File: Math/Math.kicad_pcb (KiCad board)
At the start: 2 copper layers, 100 x 100 mm, 6 parts, among them J1 Buss, U1 AM9511A, U2 74LS85, U3 74LS04, U4 74LS30

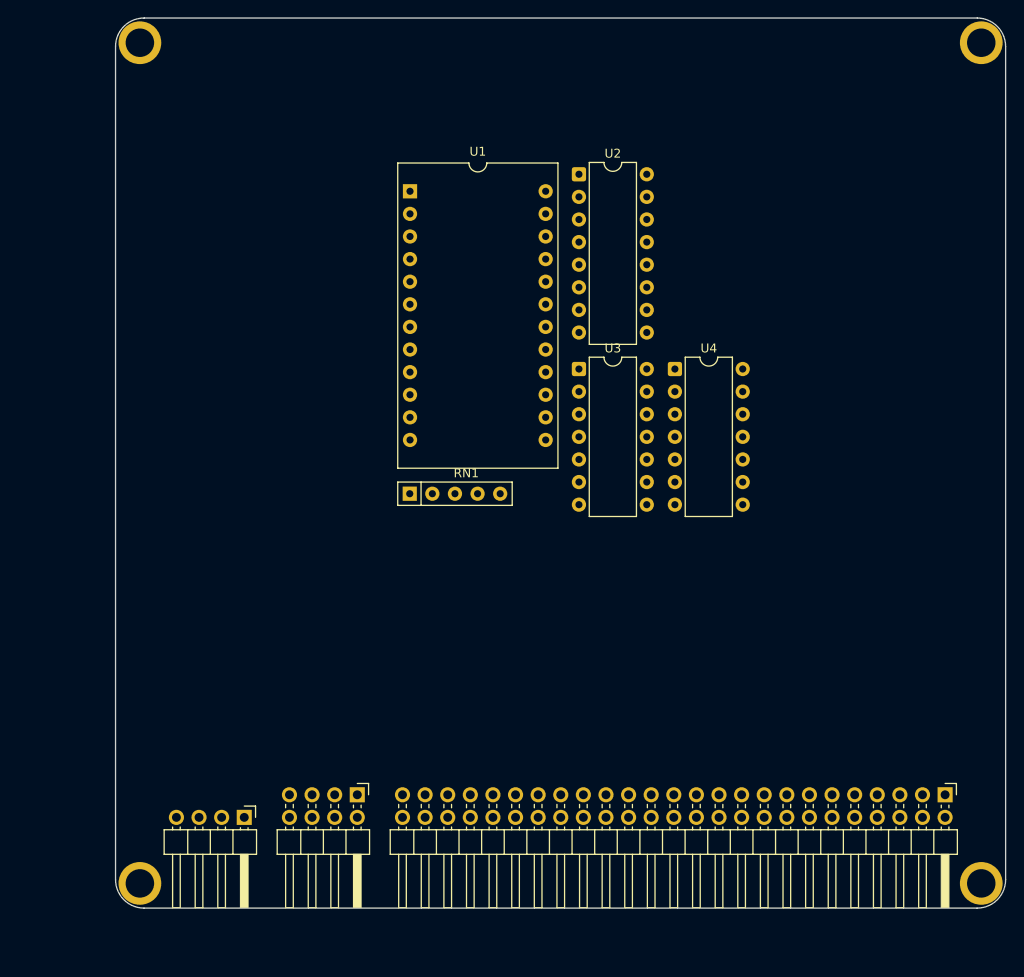
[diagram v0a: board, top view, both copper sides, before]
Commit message: mainly actually saving out vs.code along with sorting out the math card
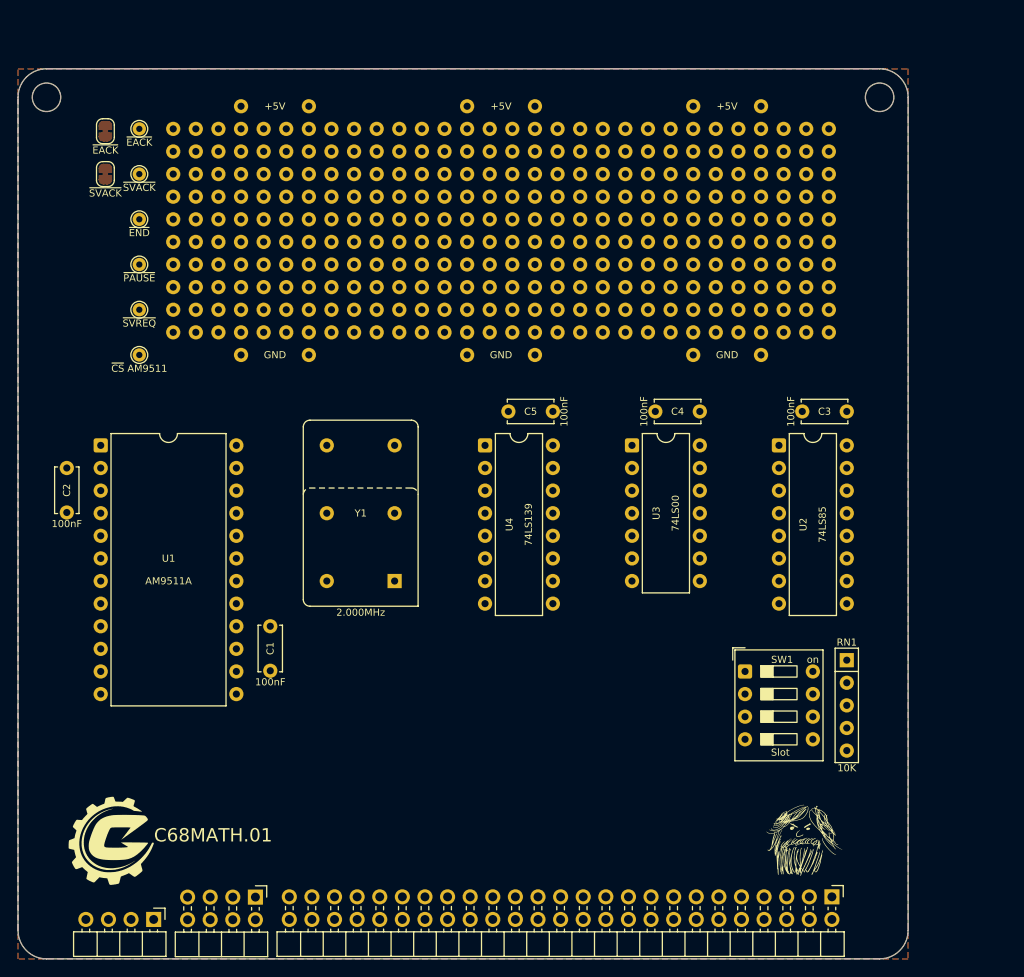
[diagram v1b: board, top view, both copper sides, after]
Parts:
- added C1: 100nF, 0-Footprints:C_Disc_D5.0mm_W2.5mm_P5.00mm, F.Cu at (53.3, 87.6)
- added C2: 100nF, 0-Footprints:C_Disc_D5.0mm_W2.5mm_P5.00mm, F.Cu at (30.5, 69.8)
- added C3: 100nF, 0-Footprints:C_Disc_D5.0mm_W2.5mm_P5.00mm, F.Cu at (118.1, 63.5)
- added C4: 100nF, 0-Footprints:C_Disc_D5.0mm_W2.5mm_P5.00mm, F.Cu at (101.6, 63.5)
- added C5: 100nF, 0-Footprints:C_Disc_D5.0mm_W2.5mm_P5.00mm, F.Cu at (80.1, 63.5)
- added G1: Logo, 0-Footprints:Crank, F.Cu at (35.6, 111.8)
- added G2: Logo, 0-Footprints:crankery_small, F.Cu at (113.0, 111.8)
- added JP1: ~{EACK}, 0-Footprints:SolderJumper-2_P1.3mm_Bridged_RoundedPad1.0x1.5mm, F.Cu at (34.8, 32.0)
- added JP2: ~{SVACK}, 0-Footprints:SolderJumper-2_P1.3mm_Bridged_RoundedPad1.0x1.5mm, F.Cu at (34.8, 36.8)
- added QC1: Grid, 0-Footprints:Grid, F.Cu at (42.4, 29.2)
- added QC2: Grid, 0-Footprints:Grid, F.Cu at (67.8, 29.2)
- added QC3: Grid, 0-Footprints:Grid, F.Cu at (93.2, 29.2)
- added SW1: Slot, 0-Footprints:SW_DIP_SPSTx04_Slide_9.78x12.34mm_W7.62mm_P2.54mm, F.Cu at (106.7, 92.7)
- added TP1: ~{EACK}, 0-Footprints:TestPoint_THTPad_D1.5mm_Drill0.7mm, F.Cu at (38.6, 31.8)
- added TP2: ~{SVACK}, 0-Footprints:TestPoint_THTPad_D1.5mm_Drill0.7mm, F.Cu at (38.6, 36.8)
- added TP3: ~{END}, 0-Footprints:TestPoint_THTPad_D1.5mm_Drill0.7mm, F.Cu at (38.6, 41.9)
- added TP4: ~{PAUSE}, 0-Footprints:TestPoint_THTPad_D1.5mm_Drill0.7mm, F.Cu at (38.6, 47.0)
- added TP5: ~{SVREQ}, 0-Footprints:TestPoint_THTPad_D1.5mm_Drill0.7mm, F.Cu at (38.6, 52.1)
- added TP6: ~{CS} AM9511, 0-Footprints:TestPoint_THTPad_D1.5mm_Drill0.7mm, F.Cu at (38.6, 57.1)
- added Y1: 2.000MHz, 0-Footprints:Oscillator_DIP-14, F.Cu at (67.3, 82.5)
- RN1: footprint Resistor_THT:R_Array_SIP5 -> 0-Footprints:R_Array_SIP5
- U1: footprint Package_DIP:DIP-24_18.0mmx34.29mm_W15.24mm -> 0-Footprints:DIP-24_W15.24mm
- U2: footprint Package_DIP:DIP-16_W7.62mm -> 0-Footprints:DIP-16_W7.62mm
- U3: value 74LS04 -> 74LS00; footprint Package_DIP:DIP-14_W7.62mm -> 0-Footprints:DIP-14_W7.62mm
- U4: value 74LS30 -> 74LS139; footprint Package_DIP:DIP-14_W7.62mm -> 0-Footprints:DIP-16_W7.62mm
- moved RN1 52.5 mm to (118.1, 91.4), turned to -90 degrees
- moved U1 45.0 mm to (34.3, 67.3)
- moved U2 37.9 mm to (110.5, 67.3)
- moved U4 23.0 mm to (77.5, 67.3)
- moved J1 12.4 mm to (25.0, 25.0)
- moved U3 10.4 mm to (94.0, 67.3)
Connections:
- J1 pad B3: /Φ2 -> unconnected-(J1-Φ2-PadB3)
- U1 pad 17: unconnected-(U1-~{PAUSE}-Pad17) -> /~{PAUSE}
- U1 pad 18: /~{CS_AM9511} -> /~{CS_9511}
- U1 pad 20: /W/~{R} -> Net-(U1-~{RD})
- U1 pad 23: /Φ2 -> Net-(U1-CLK)
- U1 pad 24: unconnected-(U1-~{END}-Pad24) -> /~{END}
- U1 pad 3: +5V -> /~{EACK}
- U1 pad 4: +5V -> /~{SVACK}
- U1 pad 5: unconnected-(U1-SVREQ-Pad5) -> /SVREQ
- U3 pad 10: unconnected-(U3-Pad10) -> /SLOT_SEL
- U3 pad 12: unconnected-(U3-Pad12) -> GND
- U3 pad 13: unconnected-(U3-Pad13) -> GND
- U3 pad 2: Net-(U1-RESET) -> /~{RESET}
- U3 pad 3: /R/~{W} -> Net-(U1-RESET)
- U3 pad 4: /W/~{R} -> /R/~{W}
- U3 pad 5: /SLOT_SEL -> /R/~{W}
- U3 pad 6: /~{SLOT_SEL} -> Net-(U1-~{RD})
- U3 pad 8: Net-(U3-Pad8) -> Net-(U4A-A1)
- U4 pad 1: /A1 -> /~{IO_SEL}
- U4 pad 10: (no net) -> unconnected-(U4B-O2-Pad10)
- U4 pad 11: Net-(U3-Pad8) -> unconnected-(U4B-O1-Pad11)
- U4 pad 12: Net-(U3-Pad8) -> /~{CS_9511}
- U4 pad 13: (no net) -> /A2
- U4 pad 14: +5V -> /A1
- U4 pad 2: /A2 -> /A3
- U4 pad 3: /A3 -> Net-(U4A-A1)
- U4 pad 4: /~{SLOT_SEL} -> Net-(U4A-O0)
- U4 pad 5: /~{IO_SEL} -> unconnected-(U4A-O1-Pad5)
- U4 pad 6: Net-(U3-Pad8) -> unconnected-(U4A-O2-Pad6)
- U4 pad 7: GND -> unconnected-(U4A-O3-Pad7)
- U4 pad 8: /~{CS_AM9511} -> GND
- U4 pad 9: (no net) -> unconnected-(U4B-O3-Pad9)
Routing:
- added copper zone on B.Cu, net GND
- added copper zone on F.Cu, net GND
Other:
- board text added: "C68MATH.01"
- board text added: "Crankery - April 2026 - Dave Hamilton"
